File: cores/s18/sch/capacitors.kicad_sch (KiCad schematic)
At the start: 96 parts

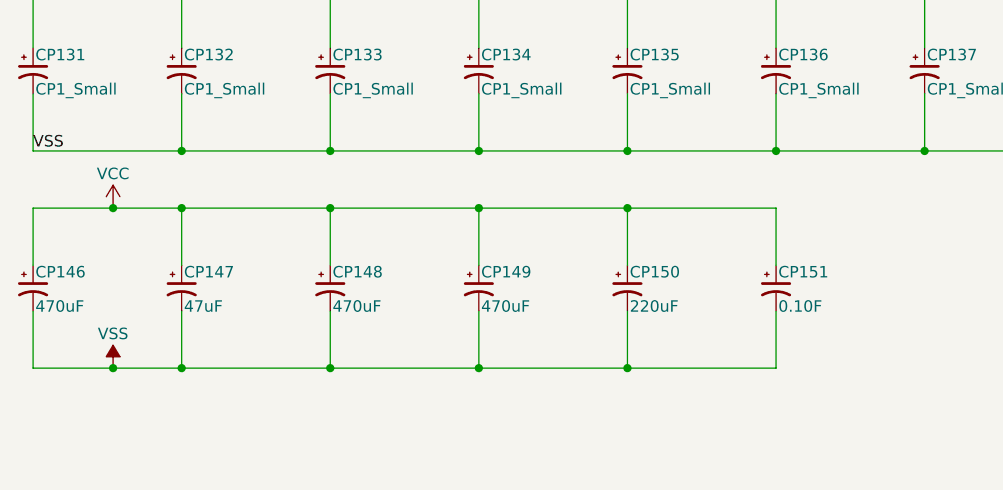
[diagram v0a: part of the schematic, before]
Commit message: system 18 schematics transferred after update
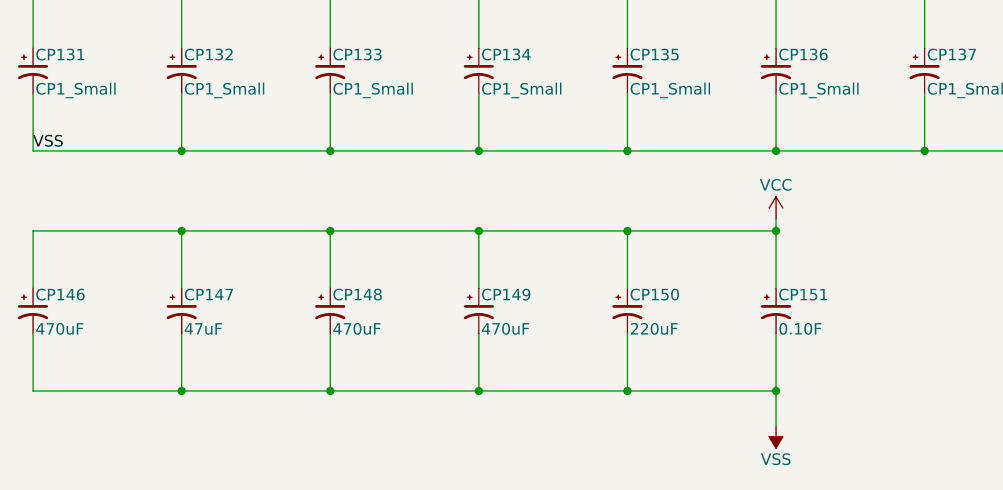
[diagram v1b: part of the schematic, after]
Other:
- moved on the sheet: CP146, CP147, CP148, CP149, CP150, CP151
